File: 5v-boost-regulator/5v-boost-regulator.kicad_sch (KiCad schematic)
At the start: 11 parts, among them J1 Conn_01x02, U1 TPS61032PWPR

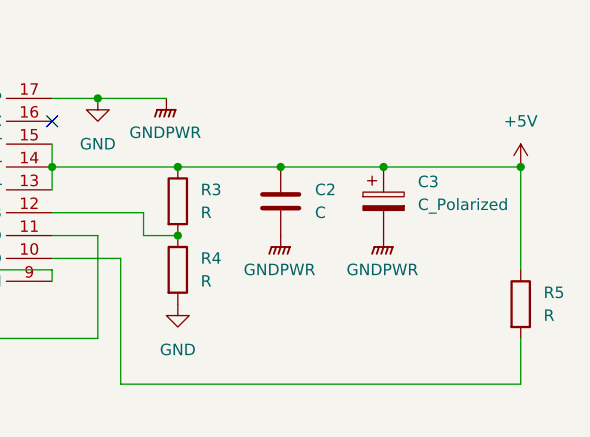
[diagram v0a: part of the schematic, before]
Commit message: update
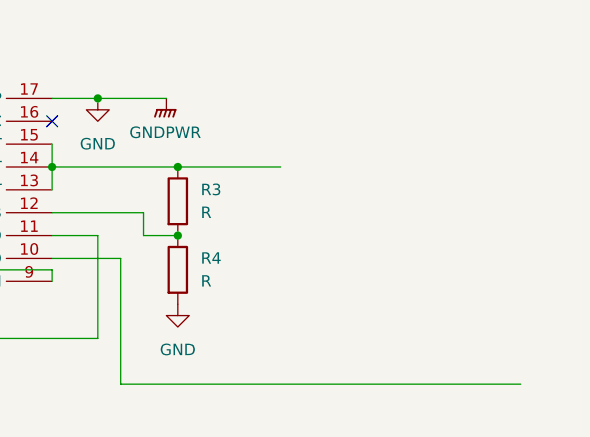
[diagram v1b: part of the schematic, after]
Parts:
- removed C2: C, Capacitor_SMD:C_1206_3216Metric, symbol Device:C
- removed C3: C_Polarized, symbol Device:C_Polarized
- removed R5: R, Resistor_SMD:R_1206_3216Metric, symbol Device:R
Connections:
- net +5V: no longer names the net of R3.1, U1.13 (VOUT), U1.14 (VOUT), U1.15 (VOUT)

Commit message: update
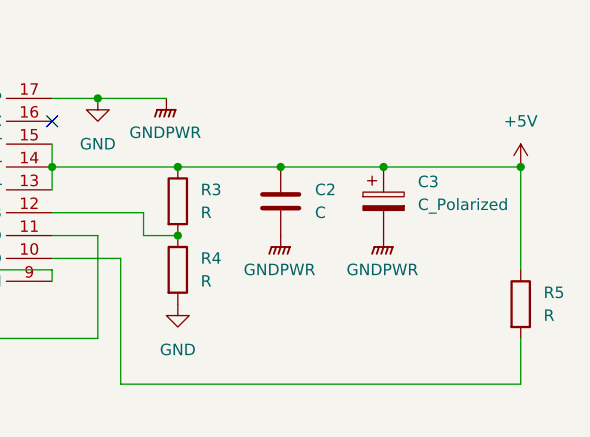
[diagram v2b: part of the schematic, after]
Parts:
- added C2: C, Capacitor_SMD:C_1206_3216Metric, symbol Device:C
- added C3: C_Polarized, symbol Device:C_Polarized
- added R5: R, Resistor_SMD:R_1206_3216Metric, symbol Device:R
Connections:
- net GND: now also C2.2, C3.2
- net +5V: now reaches R3.1, U1.13 (VOUT), U1.14 (VOUT), U1.15 (VOUT)
- net +5V: now also C2.1, C3.1, R5.1
- net at U1.10 (LBO): now also R5.2
